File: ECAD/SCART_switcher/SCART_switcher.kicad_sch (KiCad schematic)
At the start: 8 parts

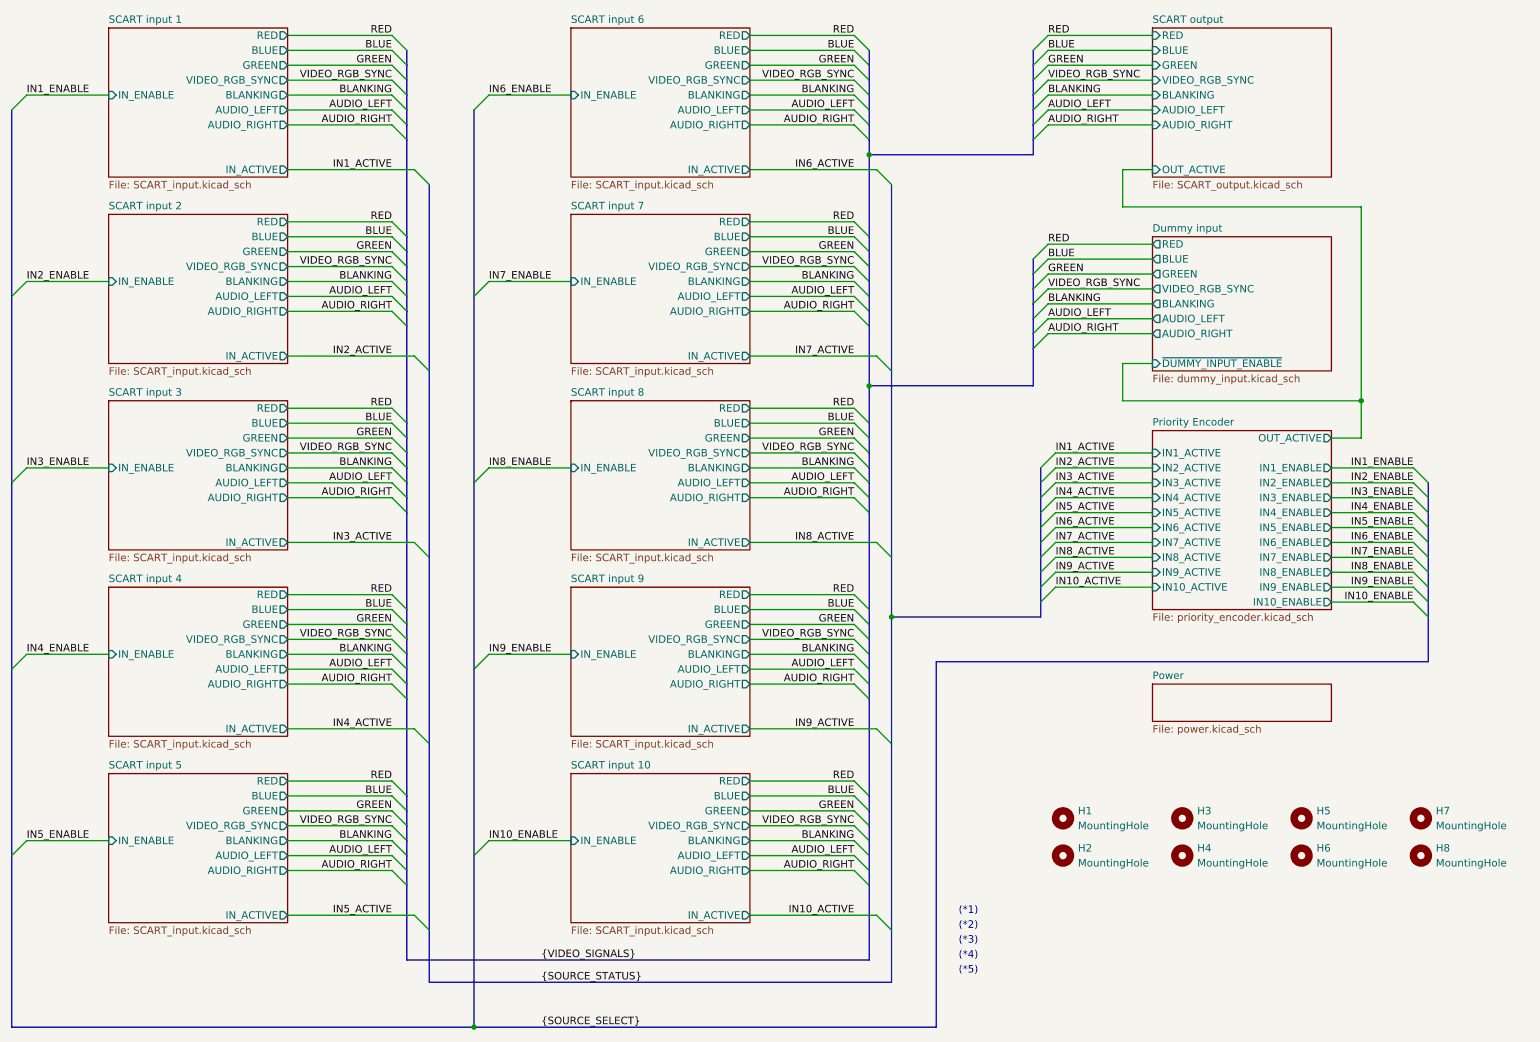
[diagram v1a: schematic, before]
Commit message: Progressed ECAD.
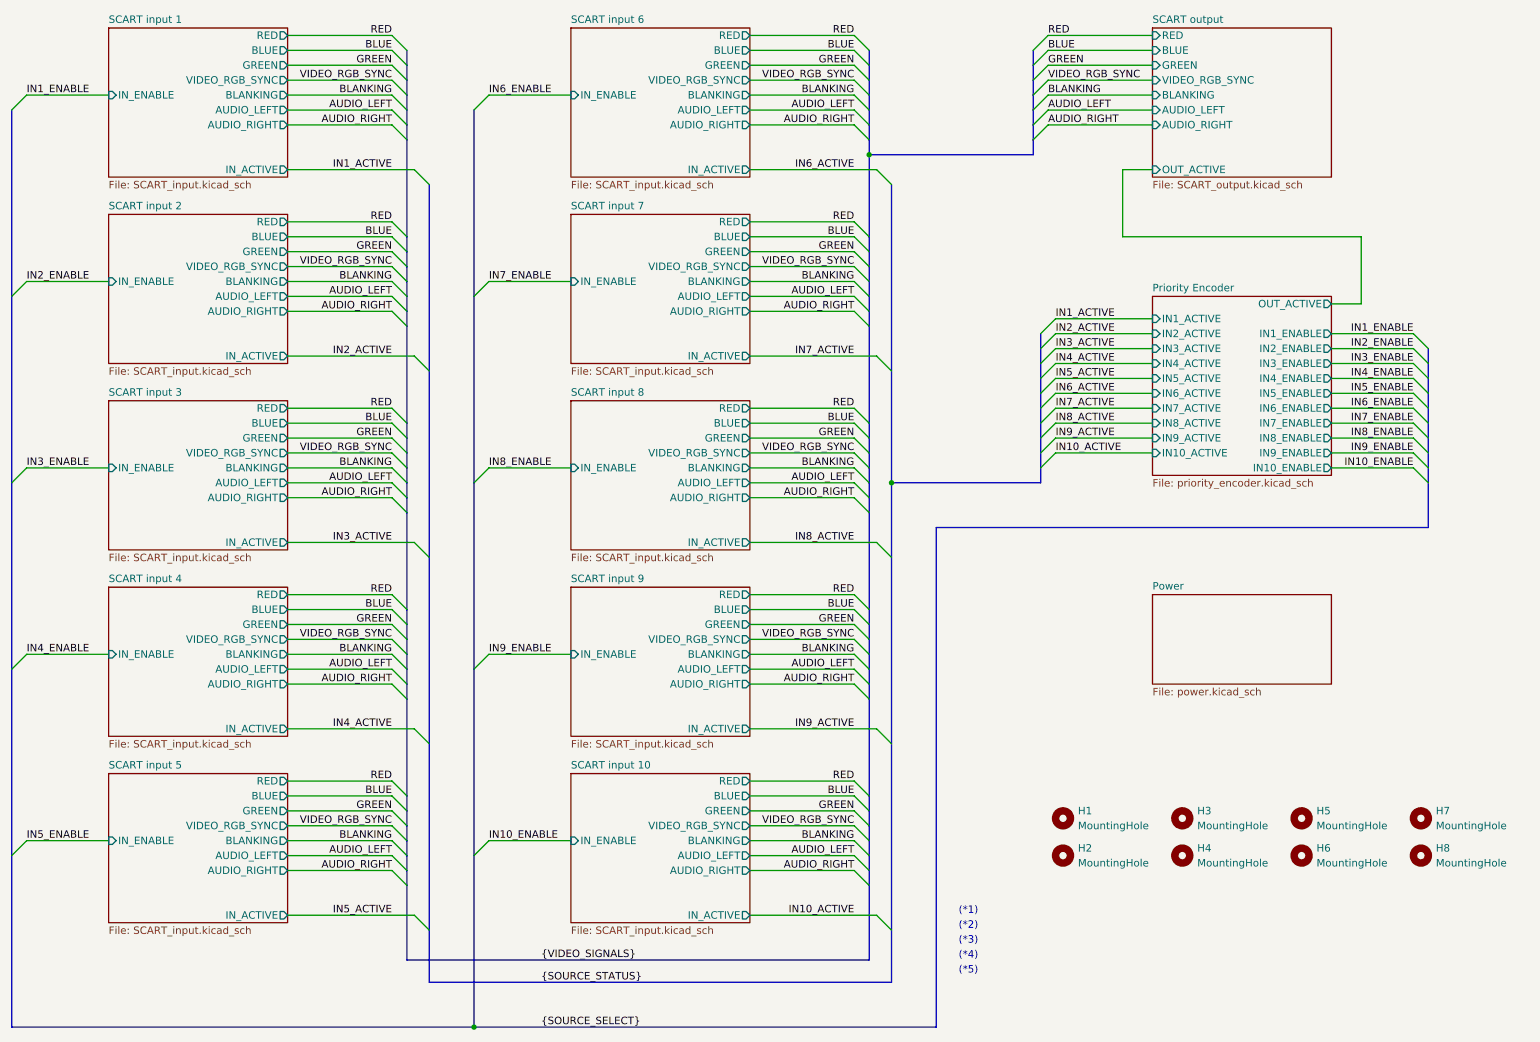
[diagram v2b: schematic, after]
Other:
- removed sheet Dummy input
